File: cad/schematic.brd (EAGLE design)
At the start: 47.5 x 32 mm, 29 parts, among them Q1 FC-255, Q2 ISP, U1 74HC595, U2 ATTINY2313, U3 PCA21125

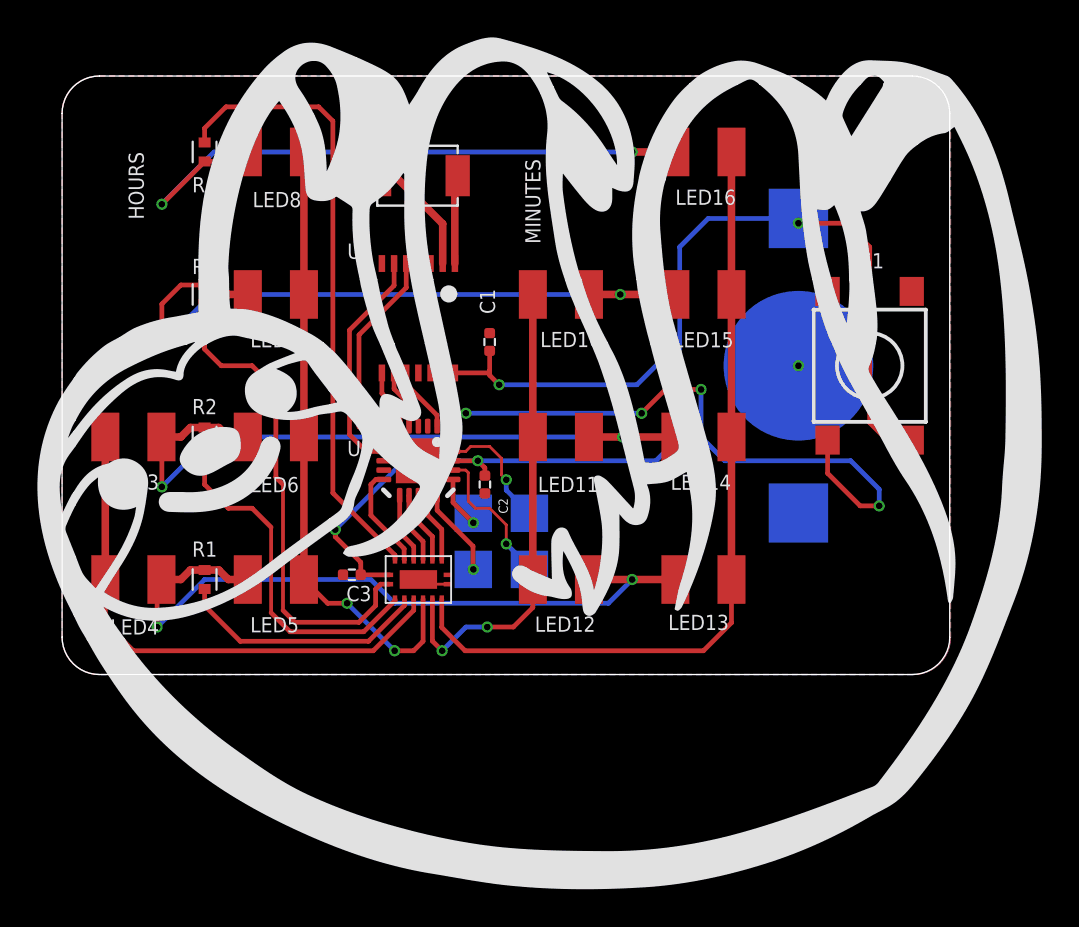
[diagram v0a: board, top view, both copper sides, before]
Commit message: update
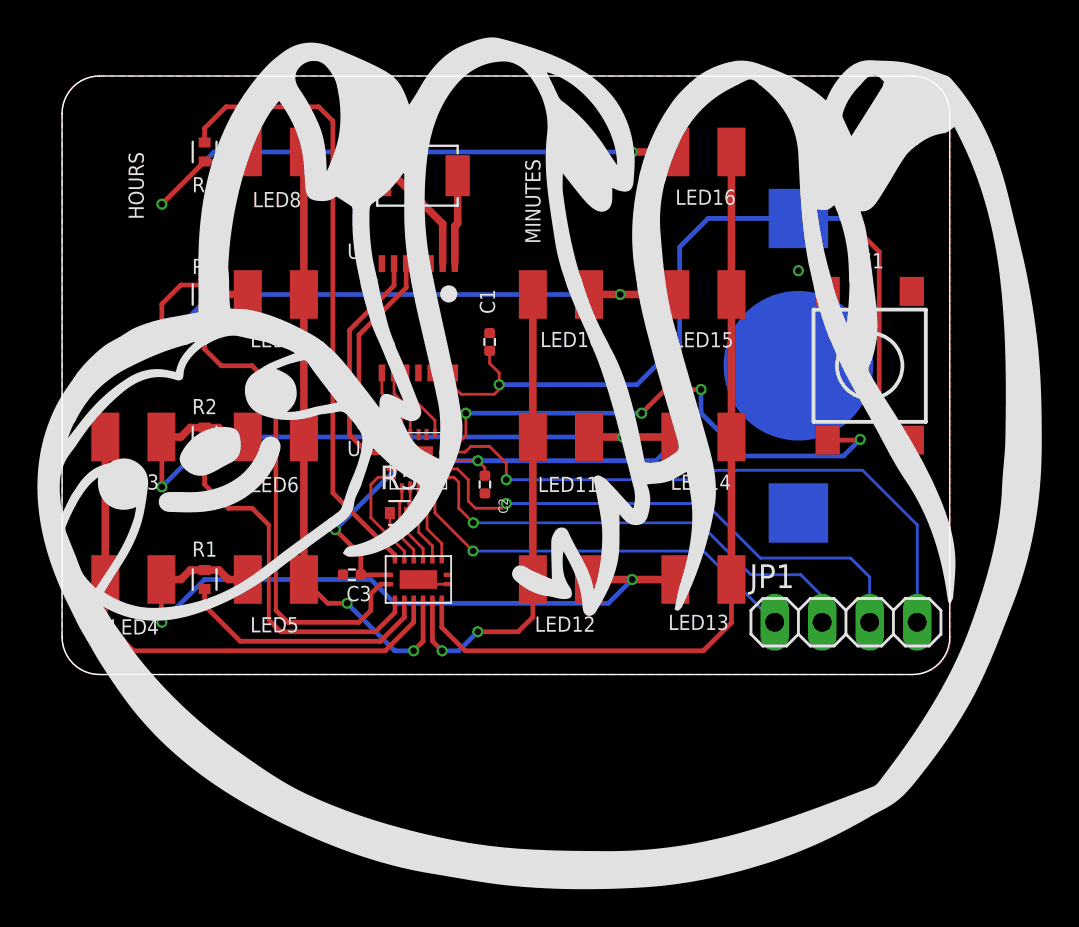
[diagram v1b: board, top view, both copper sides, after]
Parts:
- removed Q2: ISP, library:ISP
- added JP1: (no value), pinhead:1X04
- added R5: 0, Resistor:RESC1005X40
- U2: device library:MLF20-4X4 -> library:QFN20-.45MMPITCH
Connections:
- new net N$3: R5.1, U1.13
- net CLK: now also JP1.3; no longer Q2.CLK
- net GND: now also U2.21; no longer U2.TH
- net MISO: now also JP1.2; no longer Q2.MISO
- net MOSI: now also JP1.1; no longer Q2.MOSI
- net OE: now also R5.2, U2.12; no longer U1.13, U2.11
- net RST: now also JP1.4; no longer Q2.RST
- net STCP: now also U2.11; no longer U2.12
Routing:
- net RST: track 6.52 -> 33.3 mm
- net MISO: track 3.28 -> 25.0 mm
- net CLK: track 7.85 -> 28.4 mm
- net MOSI: track 4.76 -> 21.9 mm
- net BTN: track 34.5 -> 28.4 mm
- net N$3: track 0.00 -> 3.03 mm
- net OE: track 3.76 -> 1.42 mm
- net VCC: track 75.3 -> 77.6 mm
- net RR1: track 39.8 -> 39.1 mm
- net ROW2: track 18.9 -> 19.6 mm
- net STCP: track 3.77 -> 4.42 mm
